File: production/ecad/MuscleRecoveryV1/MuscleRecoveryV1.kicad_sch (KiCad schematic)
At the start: 18 parts, among them J3 Screw_Terminal_01x06, U4 ESP32-WROOM-32

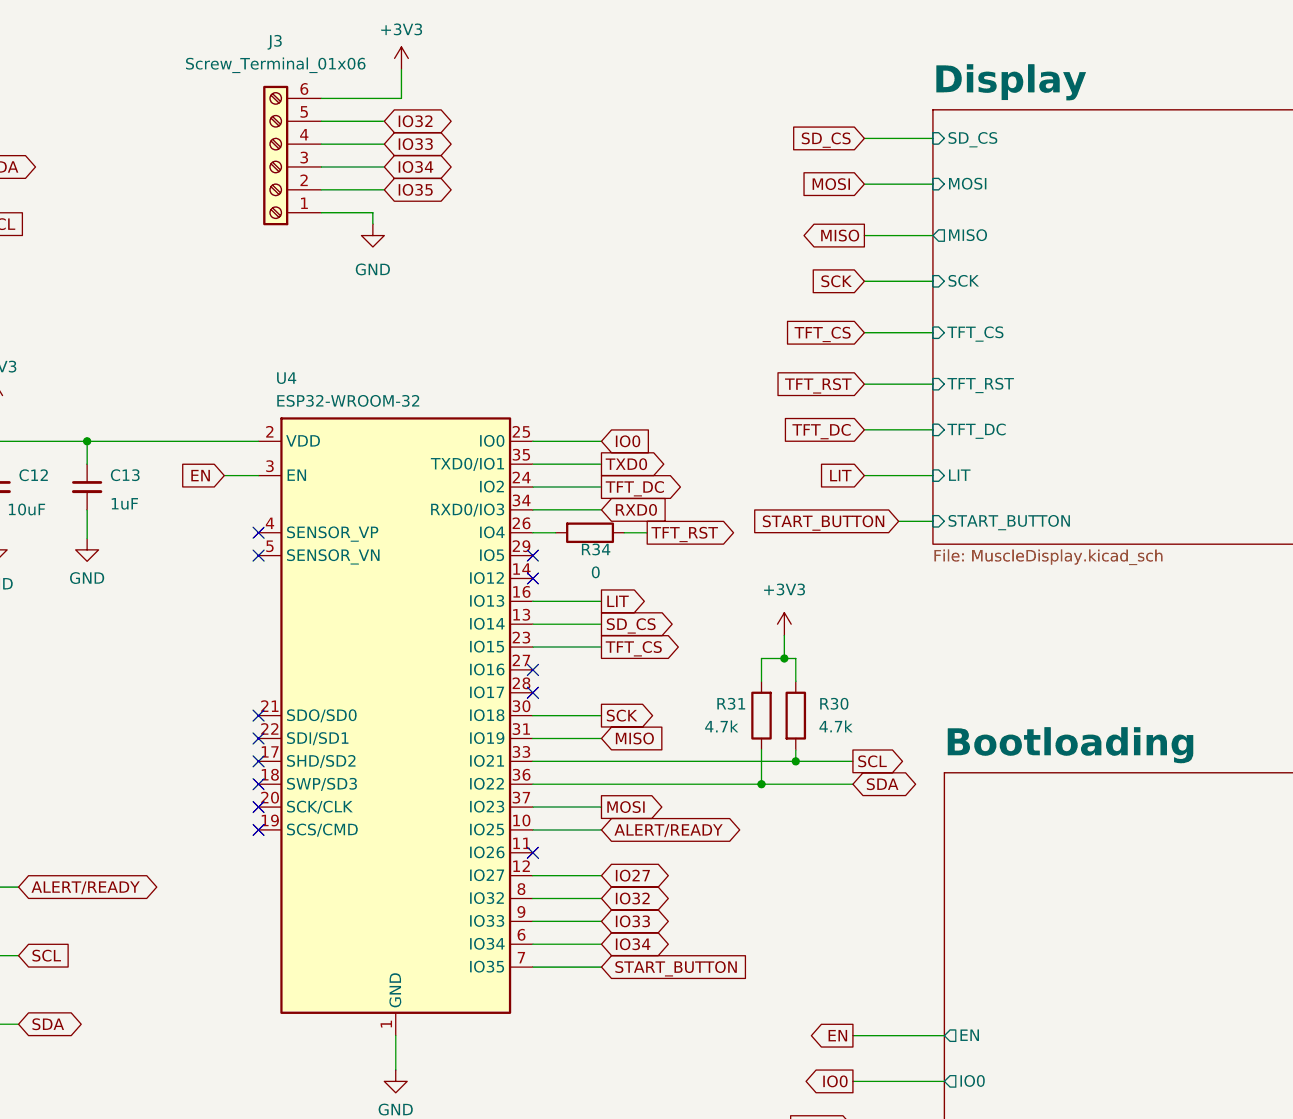
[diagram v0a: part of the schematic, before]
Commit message: Maggie fixing her mistakes lol
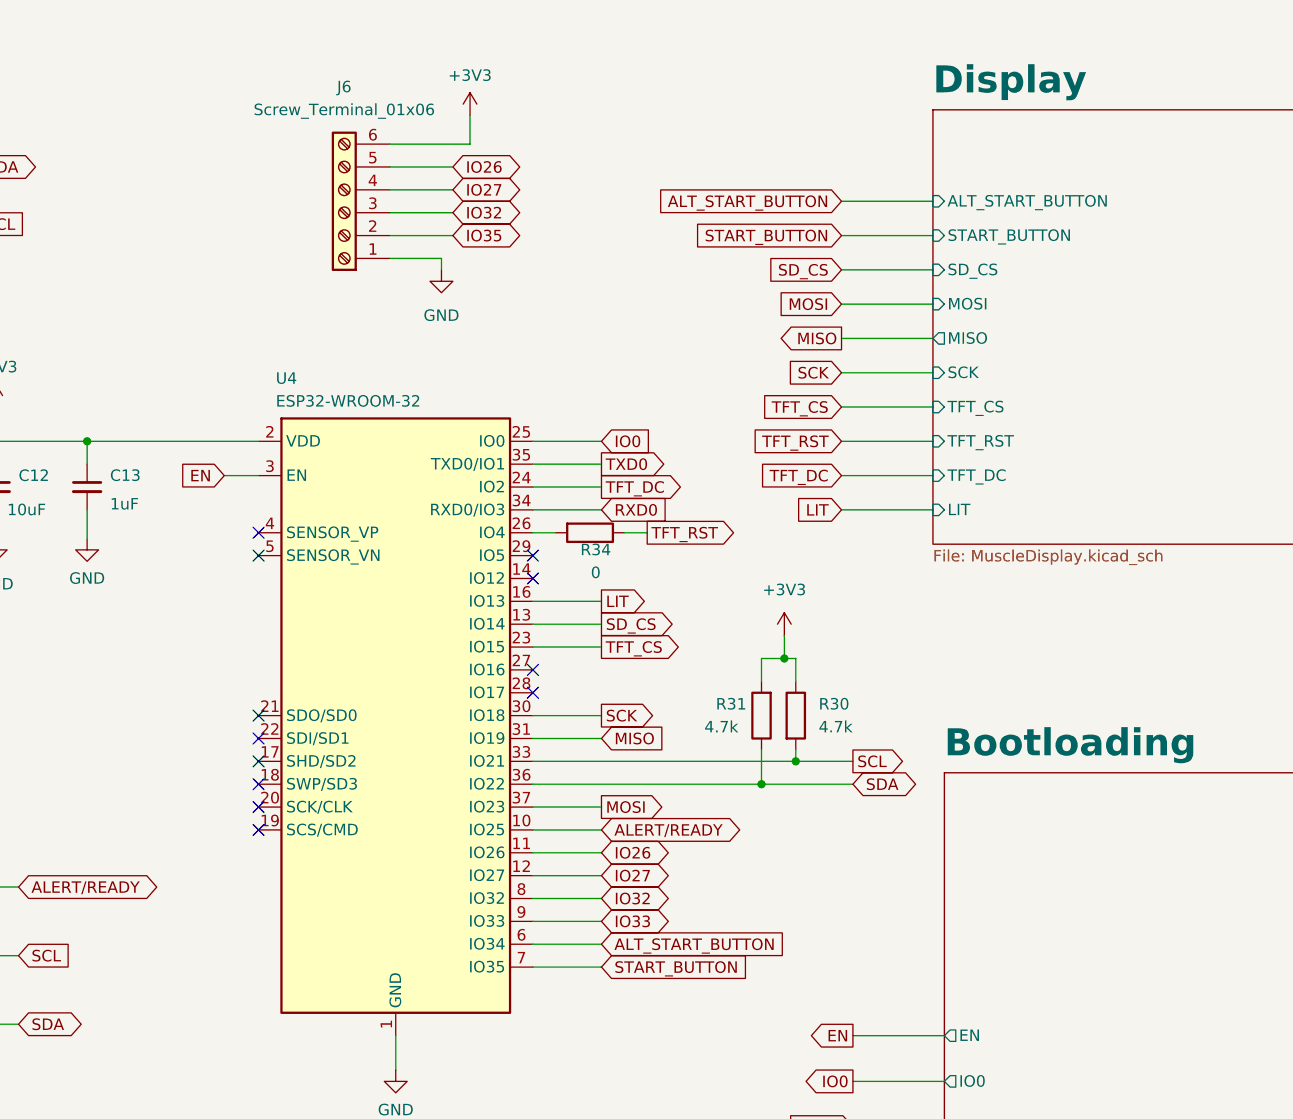
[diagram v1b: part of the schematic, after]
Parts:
- removed J3: Screw_Terminal_01x06, symbol Connector:Screw_Terminal_01x06
- added J6: Screw_Terminal_01x06, symbol Connector:Screw_Terminal_01x06
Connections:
- net +3V3: now also J6.6 (Pin_6)
- net GND: now also J6.1 (Pin_1)
- net IO27: now also J6.4 (Pin_4)
- net IO32: now also J6.3 (Pin_3)
- net IO35: now also J6.2 (Pin_2)
- net IO26: now reaches U4.11 (IO26)
- net IO26: now also J6.5 (Pin_5)
- net IO34 renamed ALT_START_BUTTON
- no-connect marks 13 -> 12
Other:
- sheet Display ports: added ALT_START_BUTTON; removed none
